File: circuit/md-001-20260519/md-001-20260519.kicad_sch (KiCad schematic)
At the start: 36 parts, among them J1 VIN-motor, J2 Conn-relay

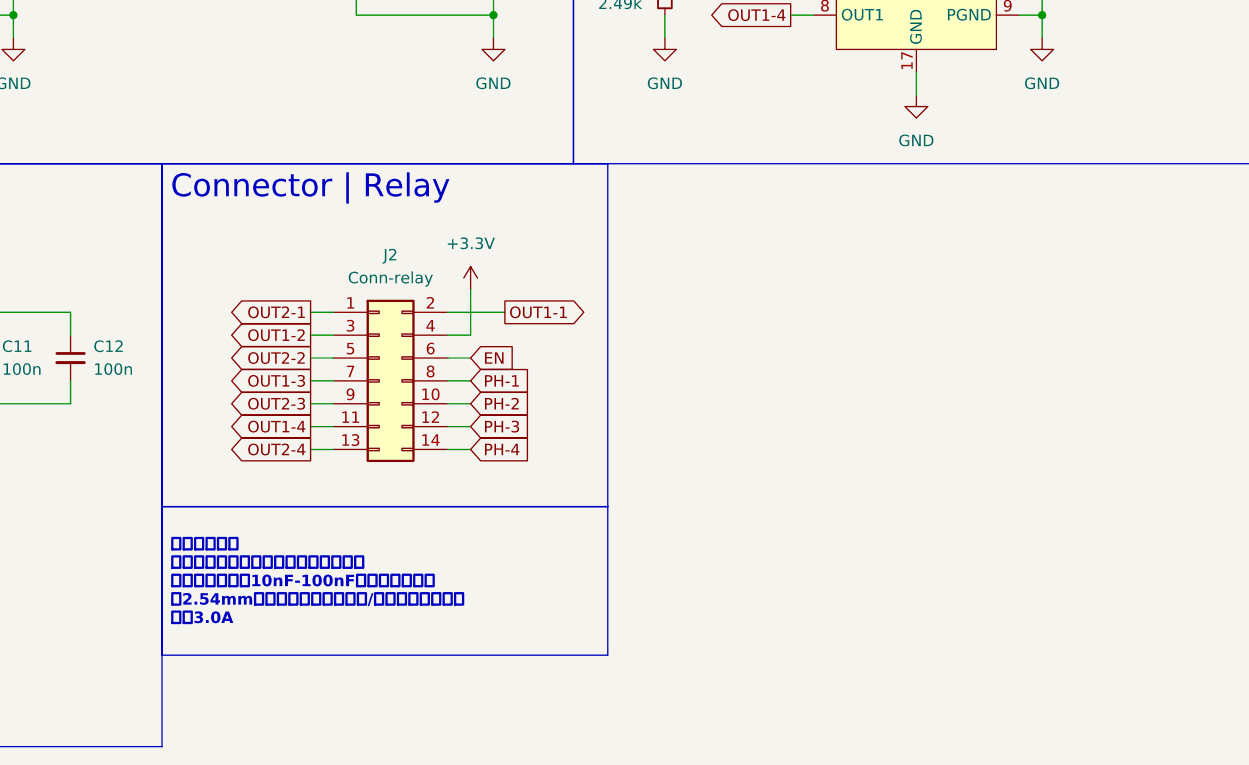
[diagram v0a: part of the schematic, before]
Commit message: Update MD基板を更新
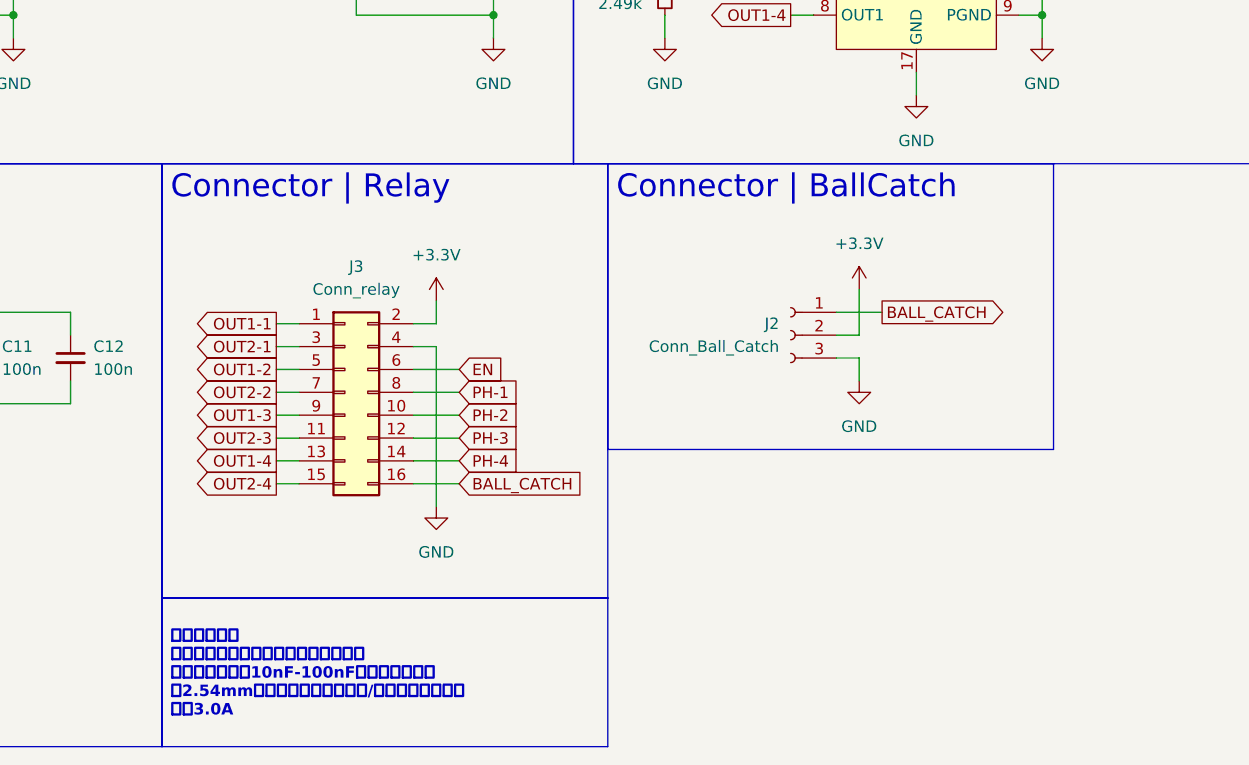
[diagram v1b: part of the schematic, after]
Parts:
- removed J2: Conn-relay, Connector_PinSocket_2.54mm:PinSocket_2x07_P2.54mm_Horizontal, symbol Connector_Generic:Conn_02x07_Odd_Even
- added J2: Conn_Ball_Catch, Connector_PinSocket_2.54mm:PinSocket_1x03_P2.54mm_Vertical, symbol Connector:Conn_01x03_Socket
- added J3: Conn_relay, Connector_PinSocket_2.54mm:PinSocket_2x08_P2.54mm_Horizontal, symbol Connector_Generic:Conn_02x08_Odd_Even
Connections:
- net +3.3V: now also J2.2 (Pin_2), J3.2 (Pin_2)
- net EN: now also J3.6 (Pin_6)
- net GND: now also J2.3 (Pin_3), J3.4 (Pin_4)
- net OUT1-1: now also J3.1 (Pin_1)
- net OUT1-2: now also J3.5 (Pin_5)
- net OUT1-3: now also J3.9 (Pin_9)
- net OUT1-4: now also J3.13 (Pin_13)
- net OUT2-1: now also J3.3 (Pin_3)
- net OUT2-2: now also J3.7 (Pin_7)
- net OUT2-3: now also J3.11 (Pin_11)
- net OUT2-4: now also J3.15 (Pin_15)
- net PH-1: now also J3.8 (Pin_8)
- net PH-2: now also J3.10 (Pin_10)
- net PH-3: now also J3.12 (Pin_12)
- net PH-4: now also J3.14 (Pin_14)
- new net BALL_CATCH: J2.1 (Pin_1), J3.16 (Pin_16)
